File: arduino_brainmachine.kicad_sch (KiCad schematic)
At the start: 86 parts, among them Q1 2N5551, Q2 2N5551, Q4 2N5551, Q5 PNP, Q6 PNP, SW1 SW_Push, U1 VOS618A, U2 VOS618A, U3 LM358_DFN, U4 LM7805_TO220

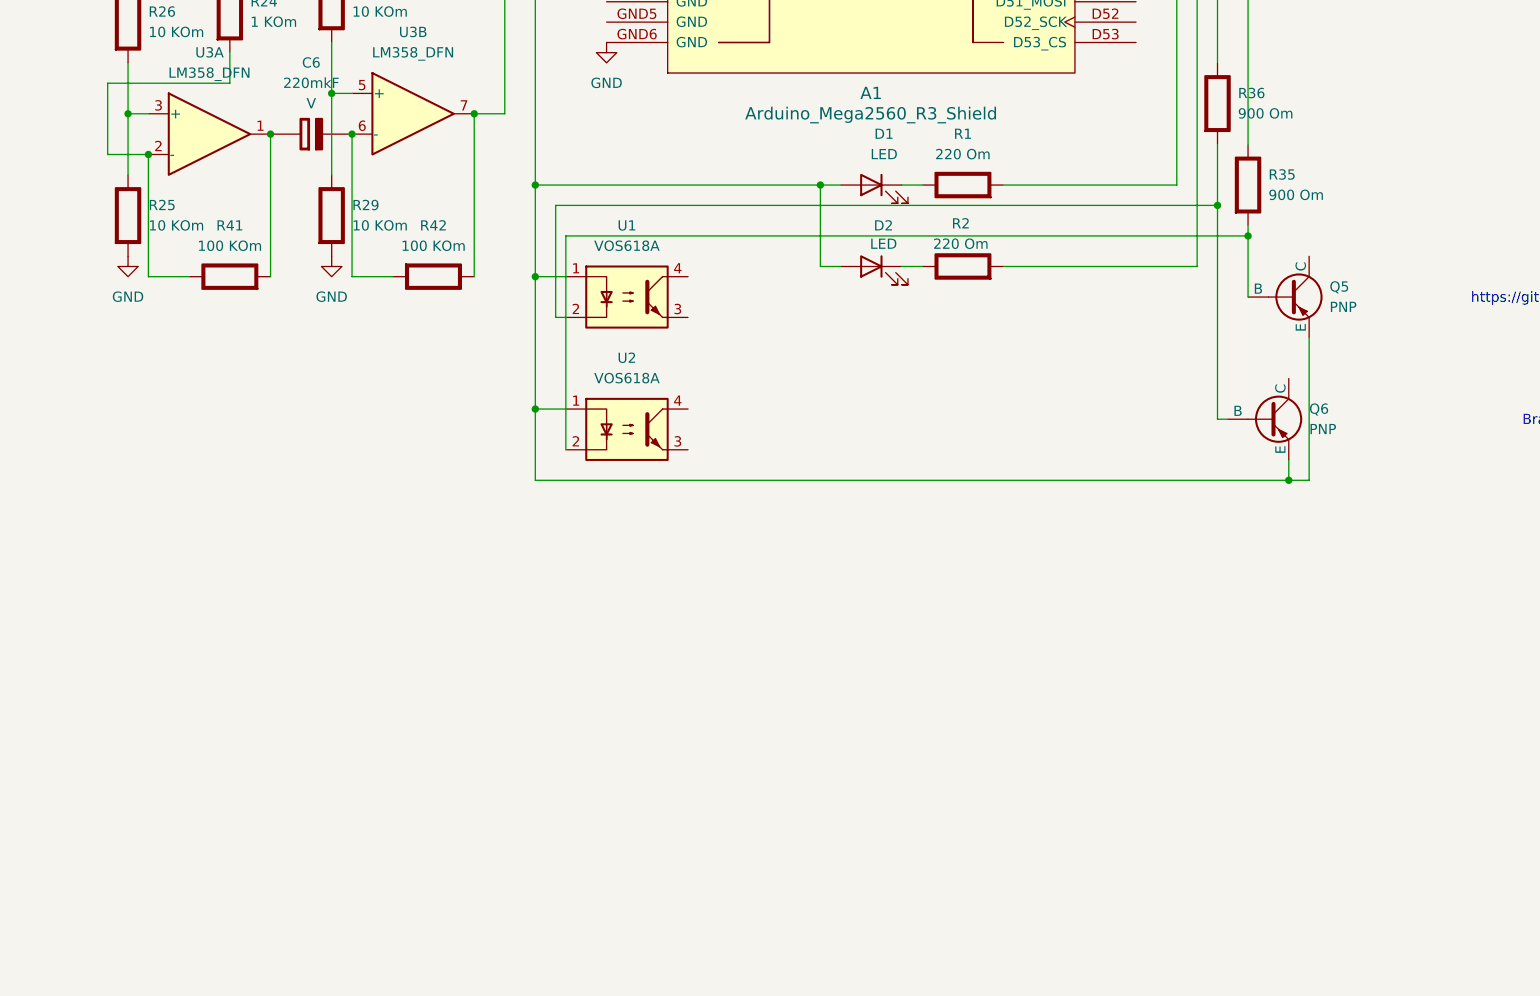
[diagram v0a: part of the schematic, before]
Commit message: Upgrade
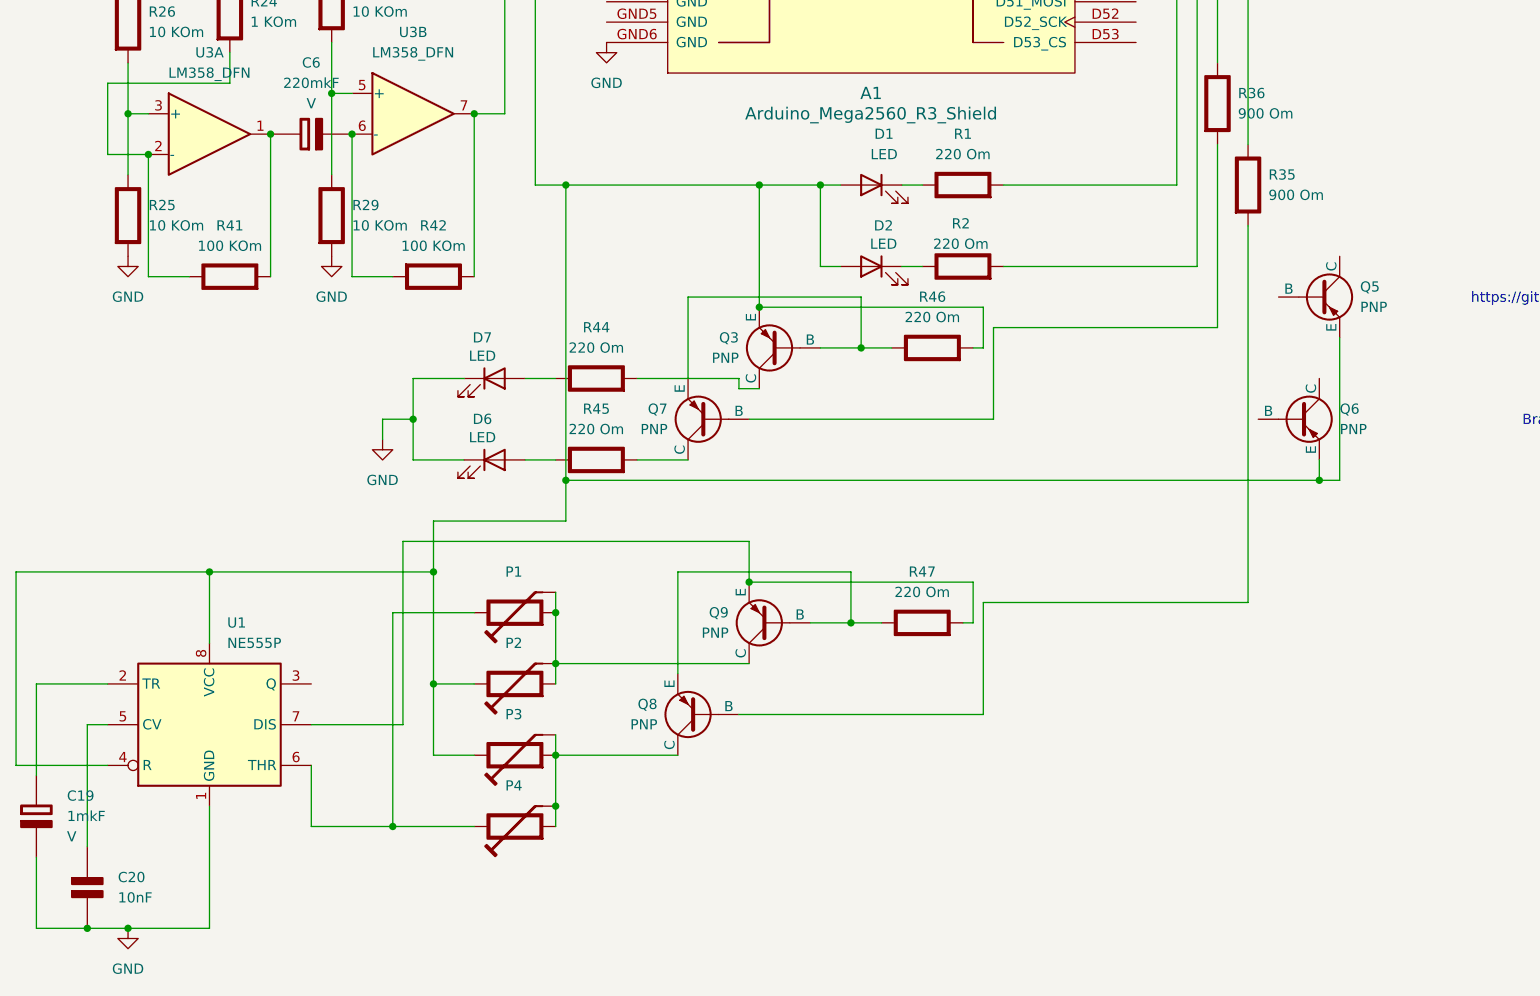
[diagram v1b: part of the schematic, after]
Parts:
- removed U1, U2: VOS618A, Package_SO:SSOP-4_4.4x2.6mm_P1.27mm, symbol Isolator:VOS618A
- added C19: 1mkF, symbol PCM_Elektuur:C-polar
- added C20: 10nF, symbol PCM_Elektuur:C
- added D6, D7: LED, symbol Device:LED
- added P1, P2, P3, P4: P-trim, symbol PCM_Elektuur:P-trim
- added Q3, Q7, Q8, Q9: PNP, symbol Simulation_SPICE:PNP
- added R44, R45, R46, R47: 220 Om, symbol PCM_Elektuur:R
- added U1: NE555P, Package_DIP:DIP-8_W7.62mm, symbol Timer:NE555P
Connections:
- net +5V: now also P2.3 (c), P3.3 (c), Q3.3 (E), R46.2 (-), U1.4 (R), U1.8 (VCC)
- net GND: now also C19.2 (-), C20.2 (-), D6.1 (K), D7.1 (K), U1.1 (GND)
- net at R36.2 (-): now also Q7.2 (B); no longer Q6.2 (B)
- net at R35.2 (-): now also Q8.2 (B); no longer Q5.2 (B)
- new net: D7.2 (A), R44.1 (+)
- new net: P3.1 (a), P3.2 (b), P4.1 (a), P4.2 (b), Q8.1 (C)
- new net: Q8.3 (E), Q9.2 (B), R47.1 (+)
- new net: Q3.1 (C), R44.2 (-)
- new net: Q9.3 (E), R47.2 (-), U1.7 (DIS)
- new net: P1.1 (a), P1.2 (b), P2.1 (a), P2.2 (b), Q9.1 (C)
- new net: Q3.2 (B), Q7.3 (E), R46.1 (+)
- new net: D6.2 (A), R45.1 (+)
- new net: Q7.1 (C), R45.2 (-)
- new net: C19.1 (+), U1.2 (TR)
- new net: P1.3 (c), P4.3 (c), U1.6 (THR)
- new net: C20.1 (+), U1.5 (CV)
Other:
- moved on the sheet: Q5, Q6

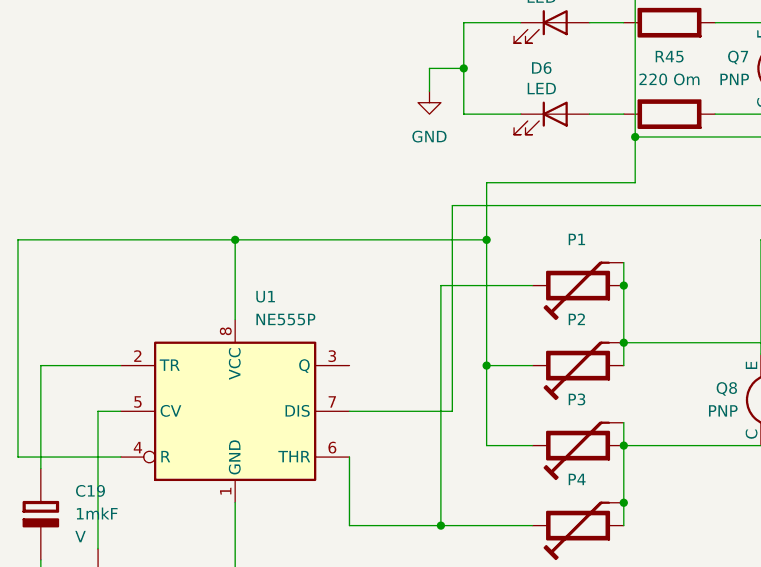
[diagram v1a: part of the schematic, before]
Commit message: Upgrade
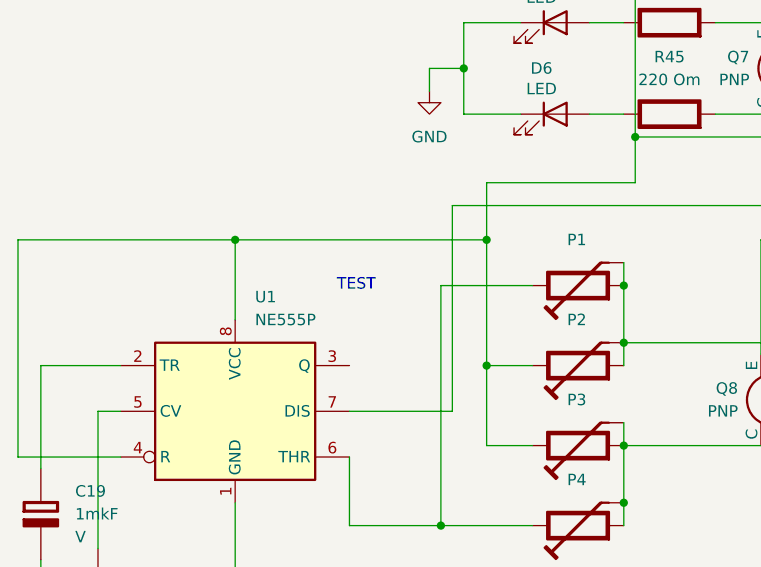
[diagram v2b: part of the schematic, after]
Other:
- note added: "TEST"
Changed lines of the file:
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@@
+		)
+	)
+	(text "TEST"
+		(exclude_from_sim no)
+		(at 42.672 213.36 0)
+		(effects
+			(font
+				(size 1.27 1.27)
+			)
 		)
 	)
